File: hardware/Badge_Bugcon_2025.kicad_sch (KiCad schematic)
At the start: 0 parts

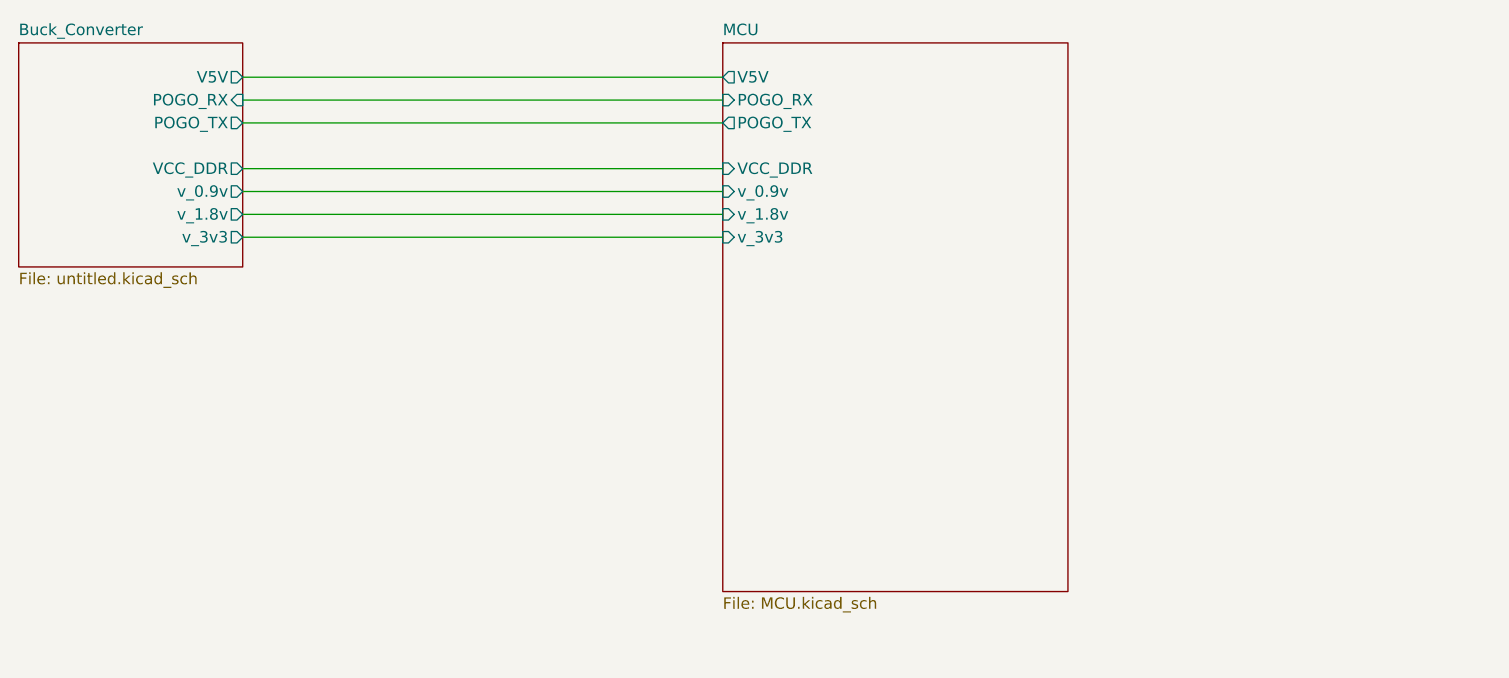
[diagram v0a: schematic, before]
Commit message: feat(Hw):Update_Schematic
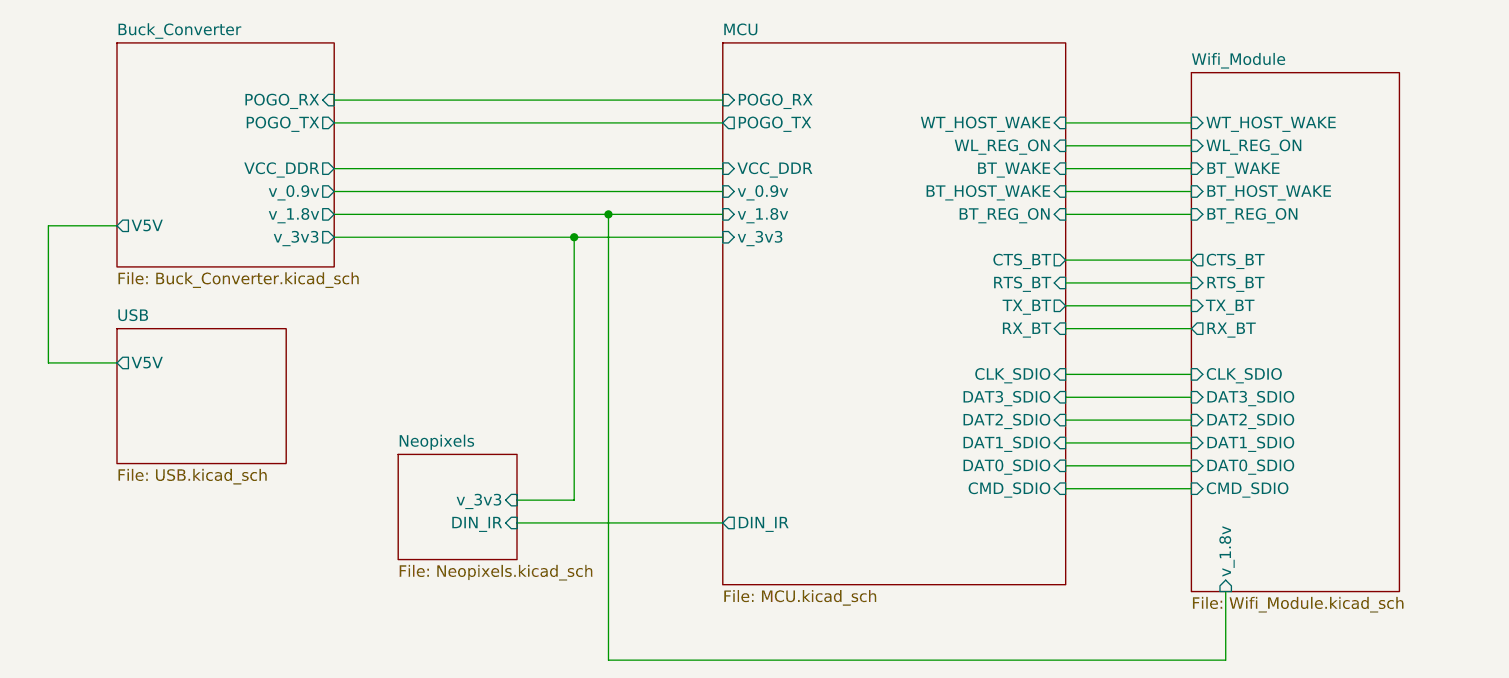
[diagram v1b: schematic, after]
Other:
- added sheet Neopixels (Neopixels.kicad_sch)
- added sheet USB (USB.kicad_sch)
- added sheet Wifi_Module (Wifi_Module.kicad_sch)
- sheet Buck_Converter: file untitled.kicad_sch -> Buck_Converter.kicad_sch
- sheet MCU ports: added BT_HOST_WAKE, BT_REG_ON, BT_WAKE, CLK_SDIO, CMD_SDIO, CTS_BT, DAT0_SDIO, DAT1_SDIO, DAT2_SDIO, DAT3_SDIO, DIN_IR, RTS_BT, RX_BT, TX_BT, WL_REG_ON, WT_HOST_WAKE; removed V5V
